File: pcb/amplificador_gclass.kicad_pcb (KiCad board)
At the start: 2 copper layers, 193.7 x 86.2 mm, 98 parts, among them J1 Jack_3.5mm_5pin, P1 CONN_01X01, P10 CONN_01X01, P12 OUT, P13 CONN_01X01, P14 MJE350, P15 MJE340, P16 2SA1302, P17 2SC3281, P18 2SC3281, P19 2SA1302, P2 CONN_01X01, P3 CONN_01X01, P4 CONN_01X01, P5 CONN_01X01, P6 CONN_01X01, P7 CONN_01X01, P8 CONN_01X01, P9 CONN_01X01, Q1 MPSA56_PNP_EBC, Q10 MPSA06_NPN_EBC, Q11 MPSA56_PNP_EBC, Q12 MPSA06_NPN_EBC, Q13 MPSA06_NPN_EBC, Q14 MPSA56_PNP_EBC, Q15 MPSA56_PNP_EBC, Q16 MPSA06_NPN_EBC, Q17 MJE340_NPN_ECB, Q18 MJE350_PNP_EBC, Q19 MJE340_NPN_ECB, Q2 MPSA56_PNP_EBC, Q20 MJE350_PNP_EBC, Q3 MPSA06_NPN_EBC, Q4 MPSA56_PNP_EBC, Q5 MPSA06_NPN_EBC, Q6 MPSA56_PNP_EBC, Q7 MPSA56_PNP_EBC, Q8 MPSA56_PNP_EBC, Q9 MPSA56_PNP_EBC

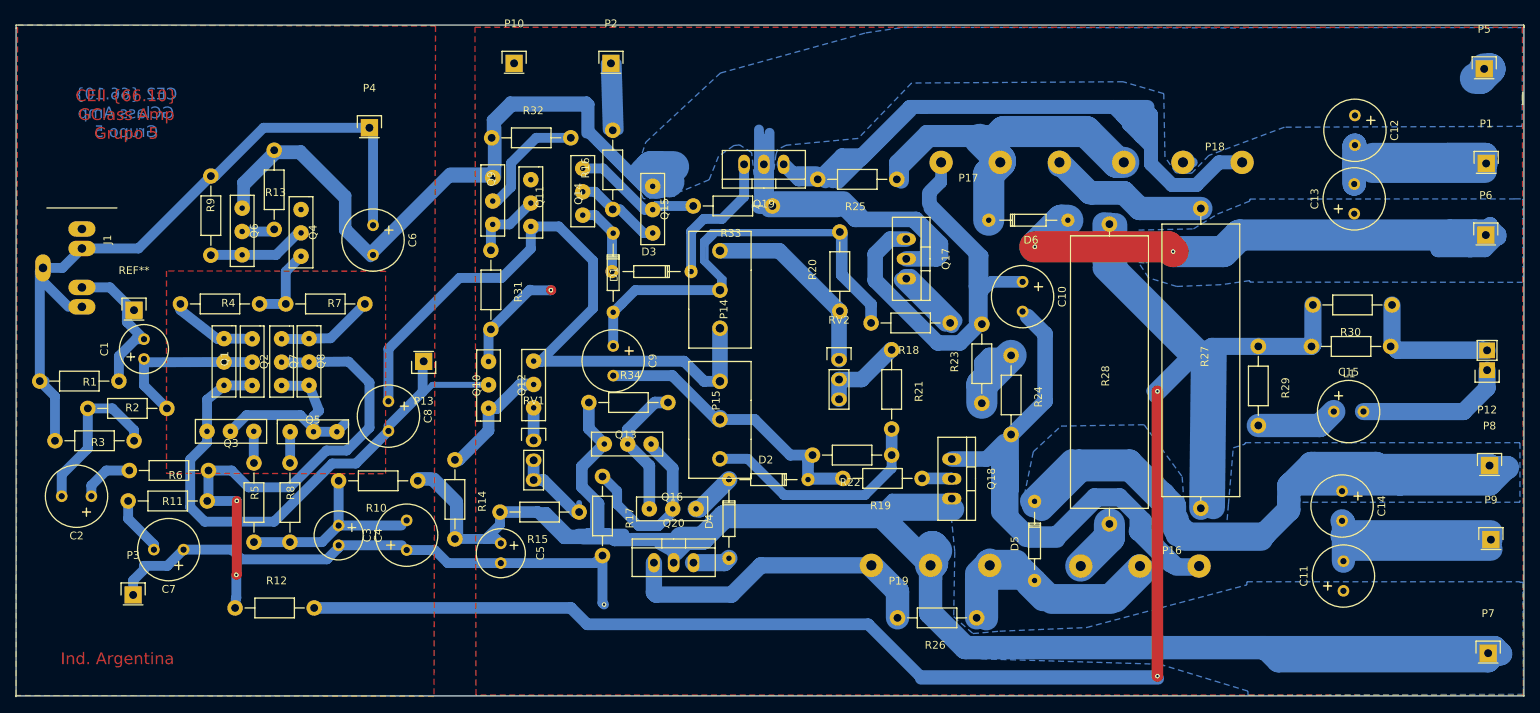
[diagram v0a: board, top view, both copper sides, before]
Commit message: Pistas MAS grandes, export archivos, arreglo pequeños defectos
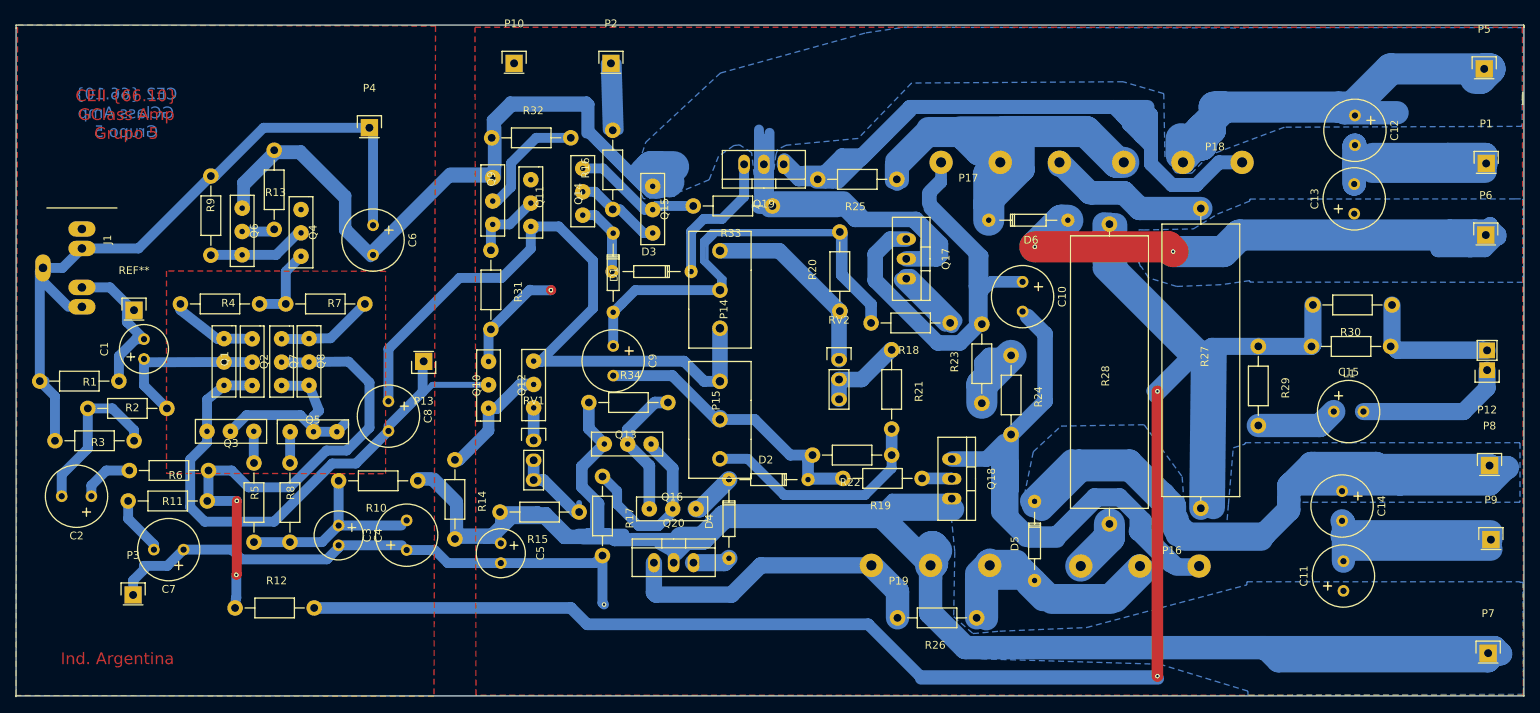
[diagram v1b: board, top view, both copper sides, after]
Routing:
- net +VA: track 290.4 -> 357.6 mm
- net Net-(D6-Pad1): track 68.0 -> 118.8 mm
- net -VA: track 352.3 -> 361.7 mm
- net Net-(P18-Pad1): track 114.1 -> 121.8 mm
- net (no net): track 20.0 -> 27.4 mm
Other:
- net class Default: trace_width 4 -> 3
